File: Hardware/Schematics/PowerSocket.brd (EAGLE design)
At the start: 100 x 47.5 mm, 74 parts, among them T1 BT138-V, T2 BT138-V, T3 BT138-V, T4 BT138-V, T5 BT138-V, T6 BT138-V

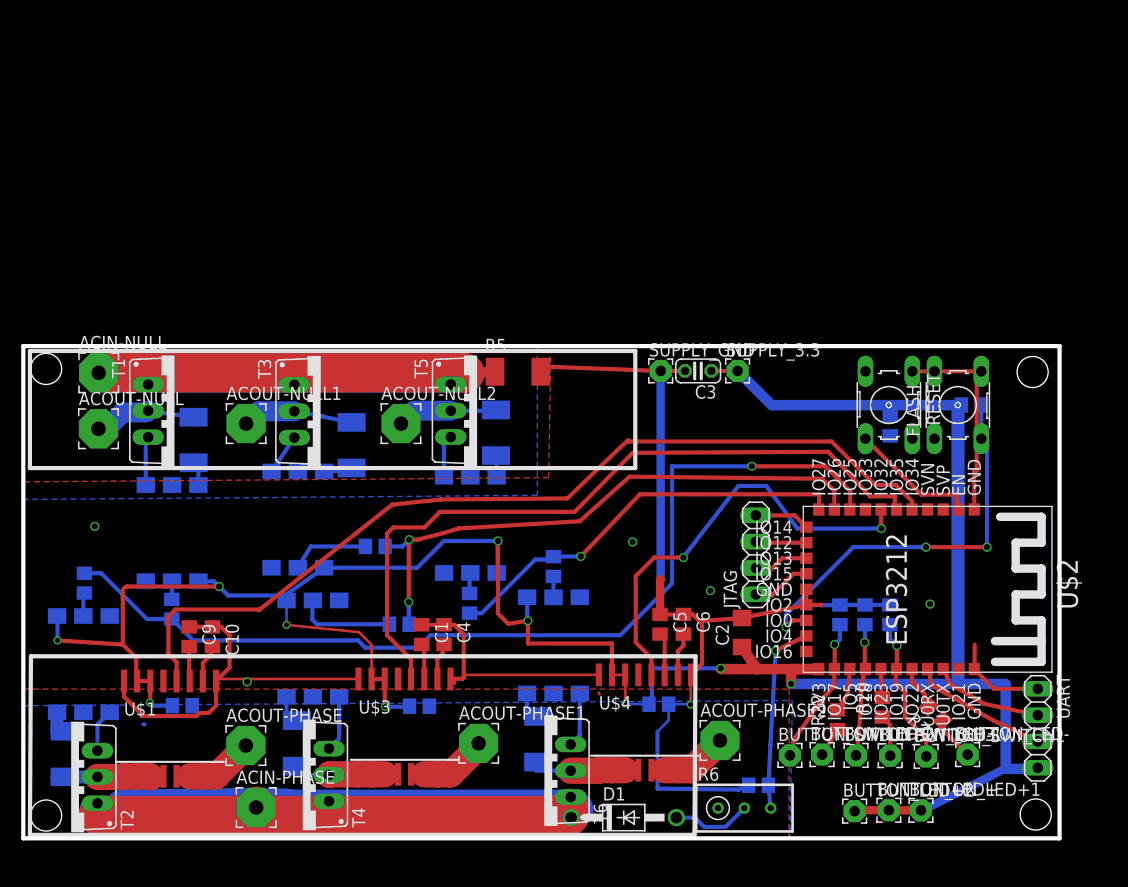
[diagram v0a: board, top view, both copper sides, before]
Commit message: New board layout
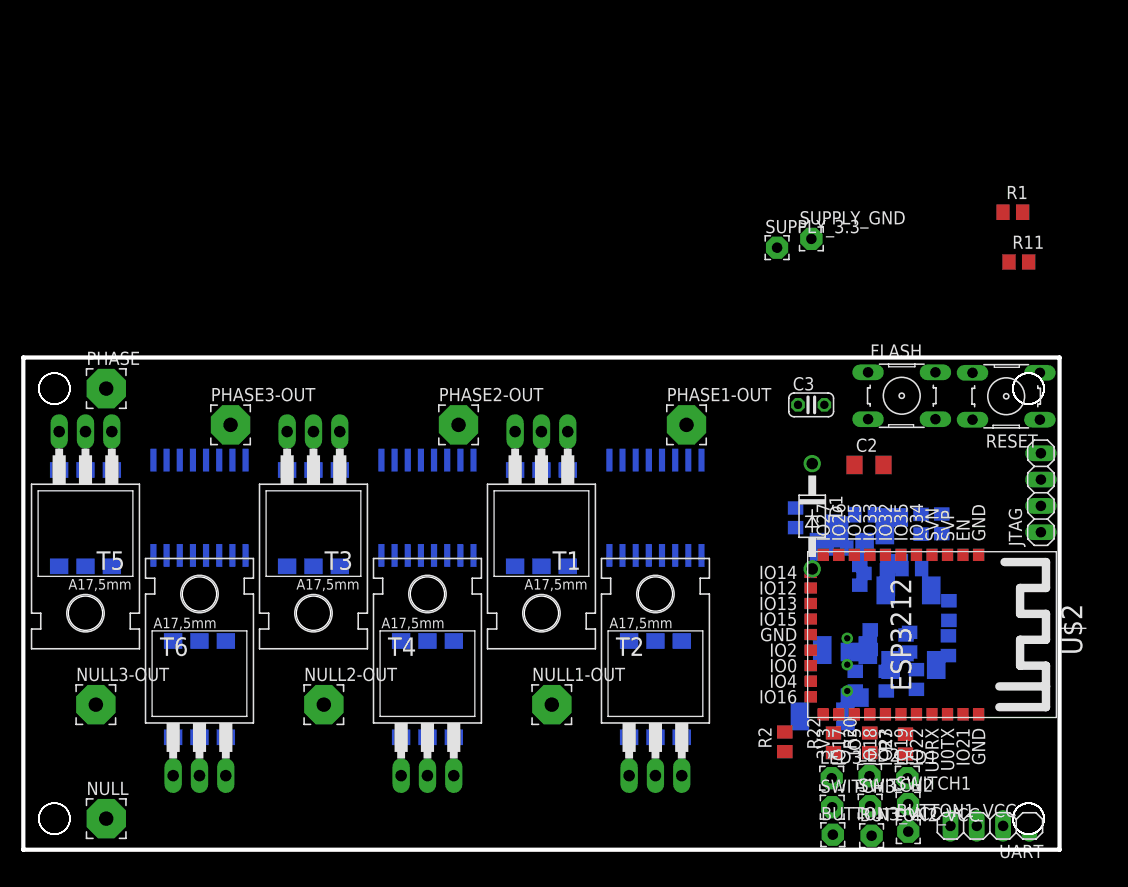
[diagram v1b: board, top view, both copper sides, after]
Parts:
- removed ACIN-NULL, ACIN-PHASE, ACOUT-NULL, ACOUT-NULL1, ACOUT-NULL2, ACOUT-PHASE, ACOUT-PHASE1, ACOUT-PHASE2: -, wirepad:3,81/1,4
- removed BUTTON_LED+: BUTTON_VCC, wirepad:2,15/1,0
- removed BUTTON_LED+1, BUTTON_LED+2, BUTTON_LED-, BUTTON_LED-1, BUTTON_LED-2, BUTTON_SWITCH1, BUTTON_SWITCH3, BUTTON_SWITCH5: -, wirepad:2,15/1,0
- removed U$1, U$3, U$4: ACS710, PowerSocket:SO-16DW
- added AMP1, AMP2, AMP3: ACS710, PowerSocket:SO-16DW
- added BUTTON1_VCC: (no value), wirepad:2,15/1,0
- added BUTTON2_VCC, BUTTON3_VCC, LED1, LED2, LED3, SWITCH1, SWITCH2, SWITCH3: -, wirepad:2,15/1,0
- added NULL, NULL1-OUT, NULL2-OUT, NULL3-OUT, PHASE, PHASE1-OUT, PHASE2-OUT, PHASE3-OUT: -, wirepad:3,81/1,4
- added R24: 0, eagle-ltspice:R2010
- R14, R18: device rcl:C0805 -> rcl:R0805
- T1, T2, T3, T4, T5, T6: value BT138-V -> BT138-H; device triac:TO220BV -> triac:TO220BH
- moved R9 83.6 mm to (89.3, 19.7), turned to 270 degrees
- moved R10 79.9 mm to (80.9, 30.8), turned to 180 degrees
- moved C11 71.6 mm to (85.7, 27.1)
- moved R3 69.1 mm to (83.4, 26.1)
- moved C10 67.3 mm to (85.5, 20.0), flipped to the bottom
- moved R4 66.1 mm to (79.3, 19.3), turned to 0 degrees
- moved C9 65.5 mm to (81.1, 27.6), flipped to the bottom
- moved T2 56.8 mm to (61.0, 13.5), turned to 0 degrees
- moved R11 56.4 mm to (96.1, 56.7), flipped to the top
- moved R15 55.9 mm to (79.0, 29.2), turned to 180 degrees
- moved R12 55.7 mm to (89.3, 23.1), turned to 270 degrees
- moved OK2 55.3 mm to (61.0, 15.5)
- moved R13 52.5 mm to (77.1, 12.9), turned to 0 degrees
- moved C1 49.3 mm to (86.6, 31.4), flipped to the bottom
- moved C4 49.2 mm to (88.6, 31.4), flipped to the bottom
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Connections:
- net N$25 renamed GATE2
- net N$3 renamed VOLTMETER
- removed net N$15 (its old number): BUTTON_LED-.1, R7.1
- removed net N$2 (its old number): R1.1, RESET.4, U$2.EN
- removed net N$36 (its old number): ACOUT-PHASE1.1, U$3.5, U$3.6, U$3.7, U$3.8
- removed net N$40: U$3.13
- removed net N$42 (its old number): OK5.2, R16.2
- removed net N$43: OK5.6, R17.1
- removed net N$45: ACIN-NULL.1, R5.1, T1.T1, T3.T1, T5.T1
- removed net N$46: OK6.2, R18.1
- removed net N$47: OK6.6, R19.1
- removed net N$49: R19.2, T6.T2, U$4.1, U$4.2, U$4.3, U$4.4
- removed net N$50: U$4.13
- removed net N$51: ACIN-PHASE.1, D1.C, T2.T1, T4.T1, T6.T1
- removed net N$52: R22.2, U$2.IO5
- removed net N$53: R15.2, T4.T2, U$3.1, U$3.2, U$3.3, U$3.4
- removed net N$54: R16.1, R18.2, U$2.IO27
- removed net N$55: C9.2, U$1.11
- removed net N$60: C10.2, U$1.10
- removed net N$62: C1.2, U$3.11
- removed net N$63: C4.2, U$3.10
- removed net N$64: C5.2, U$4.11
- removed net N$65: C6.2, U$4.10
- new net AMP1: AMP1.12, U$2.IO34
- new net AMP2: AMP2.12, U$2.IO35
- new net AMP3: AMP3.12, U$2.IO32
- new net BUTTON1: R8.1, SWITCH1.1, U$2.IO22
- new net BUTTON2: R21.1, SWITCH2.1, U$2.IO23
- new net BUTTON3: R23.1, SWITCH3.1, U$2.IO5
- new net GATE1: R3.2, R9.2, U$2.IO25
- new net GATE3: R16.1, R18.1, U$2.IO27
- new net LED1: R7.2, U$2.IO19
- new net LED2: R20.2, U$2.IO18
- new net LED3: R22.2, U$2.IO17
- new net N$24: FLASH.3, FLASH.4, R2.2, U$2.IO0
- new net N$30: AMP2.10, C4.1
- new net N$66: R1.1, RESET.3, RESET.4, U$2.EN
- new net NULL: NULL.1, R5.1, T2.T1, T4.T1, T6.T1
- new net PHASE: PHASE.1, R24.2, T1.T1, T3.T1, T5.T1
- new net PHASE1: AMP1.1, AMP1.2, AMP1.3, AMP1.4, R10.2, T1.T2
- new net PHASE2: AMP2.1, AMP2.2, AMP2.3, AMP2.4, R15.2, T3.T2
- new net PHASE3: AMP3.1, AMP3.2, AMP3.3, AMP3.4, R19.2, T5.T2
- net GND: now also AMP1.16, AMP1.9, AMP2.16, AMP2.9, AMP3.16, AMP3.9, C1.2, C10.2, C11.2, C12.2, C13.2, C4.2, C5.2, C6.2, C9.2, FLASH.1, R21.2, R23.2, R8.2, RESET.2; no longer C1.1, C10.1, C11.1, C12.1, C13.1, C4.1, C5.1, C6.1, C9.1, R21.1, R23.1, R8.1, U$1.16, U$1.9, U$3.16, U$3.9, U$4.16, U$4.9
- net N$1: now also OK1.2, R9.1; no longer ACOUT-NULL.1, R4.2, T1.T2
- net N$10: now also AMP3.5, AMP3.6, AMP3.7, AMP3.8, PHASE3-OUT.1; no longer OK2.2, R9.1
- net N$11: now also LED3.1, R22.1; no longer U$2.IO35, U$3.12
- net N$12: now also AMP1.10, C10.1; no longer U$1.12, U$2.IO34
- net N$13: now also AMP1.11, C9.1; no longer ACOUT-PHASE.1, U$1.5, U$1.6, U$1.7, U$1.8
- net N$14: now also NULL2-OUT.1, T4.T2; no longer ACOUT-NULL1.1, T3.T2
- net N$16: now also OK4.6, R13.1; no longer BUTTON_LED-1.1, R20.1
- net N$17: now also NULL1-OUT.1, R4.2, T2.T2; no longer BUTTON_SWITCH1.1, R8.2, U$2.IO19
- net N$18: now also OK5.2, R18.2; no longer OK1.6, R4.1
- net N$20: now also OK1.6, R10.1; no longer BUTTON_SWITCH3.1, R21.2, U$2.IO18
- net N$21: now also R4.1; no longer R10.1
- net N$23: now also OK3.6, R15.1; no longer R10.2, T2.T2, U$1.1, U$1.2, U$1.3, U$1.4
- net N$26: now also AMP2.5, AMP2.6, AMP2.7, AMP2.8, PHASE2-OUT.1; no longer BUTTON_LED-2.1, R22.1
- net N$27: now also AMP1.5, AMP1.6, AMP1.7, AMP1.8, PHASE1-OUT.1; no longer U$1.13
- net N$28: now also R14.1; no longer R12.2
- net N$29: now also OK4.2, R12.2; no longer OK3.6, R13.1
- net N$31: now also OK6.2, R16.2; no longer R20.2, U$2.IO23
- net N$32: now also AMP2.11, C1.1; no longer OK4.2, R14.1
- net N$33: now also OK6.6, R17.1; no longer OK4.6, R15.1
- net N$35: now also OK5.6, R19.1; no longer ACOUT-PHASE2.1, U$4.5, U$4.6, U$4.7, U$4.8
- net N$38: now also AMP3.10, C6.1; no longer ACOUT-NULL2.1, R17.2, T5.T2
- net N$39: now also AMP3.11, C5.1; no longer BUTTON_SWITCH5.1, R23.2, U$2.IO17
- net N$41: now also D1.C, R24.1; no longer U$2.IO32, U$4.12
- net N$6: now also OK2.2, R3.1; no longer OK1.2, R3.2
- net N$7: now also LED2.1, R20.1; no longer FLASH.3, R2.2, U$2.IO0
- net N$8: now also NULL3-OUT.1, R17.2, T6.T2; no longer R3.1, R9.2, U$2.IO25
- net N$9: now also LED1.1, R7.1; no longer R7.2, U$2.IO22
- net VCC: now also AMP1.14, AMP1.15, AMP2.14, AMP2.15, AMP3.14, AMP3.15, BUTTON1_VCC.1, BUTTON2_VCC.1, BUTTON3_VCC.1, C11.1, C12.1, C13.1; no longer BUTTON_LED+.1, BUTTON_LED+1.1, BUTTON_LED+2.1, C11.2, C12.2, C13.2, U$1.14, U$1.15, U$3.14, U$3.15, U$4.14, U$4.15
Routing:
- net VCC: track 252.8 -> 0.00 mm, vias 10 -> 0
- net GND: track 181.0 -> 0.00 mm, vias 6 -> 0
- net N$8: track 93.5 -> 0.00 mm, vias 1 -> 0
- net N$12: track 87.8 -> 0.00 mm
- net N$11: track 70.5 -> 0.00 mm
- net N$45: track 59.3 -> 0.00 mm
- net N$51: track 58.8 -> 0.00 mm
- net GATE2: track 55.9 -> 0.00 mm, vias 2 -> 0
- net N$68: track 47.4 -> 0.00 mm
- net N$41: track 41.9 -> 0.00 mm, vias 2 -> 0
- net N$54: track 40.1 -> 0.00 mm, vias 1 -> 0
- net N$7: track 39.8 -> 0.00 mm, vias 3 -> 0
- net N$37: track 34.3 -> 0.00 mm
- net VOLTMETER: track 18.5 -> 0.00 mm, vias 1 -> 0
- net N$17: track 14.2 -> 0.00 mm, vias 1 -> 0
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- removed copper zone on layer 1, net GND
- removed copper zone on layer 16, net GND

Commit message: Added .brd script.
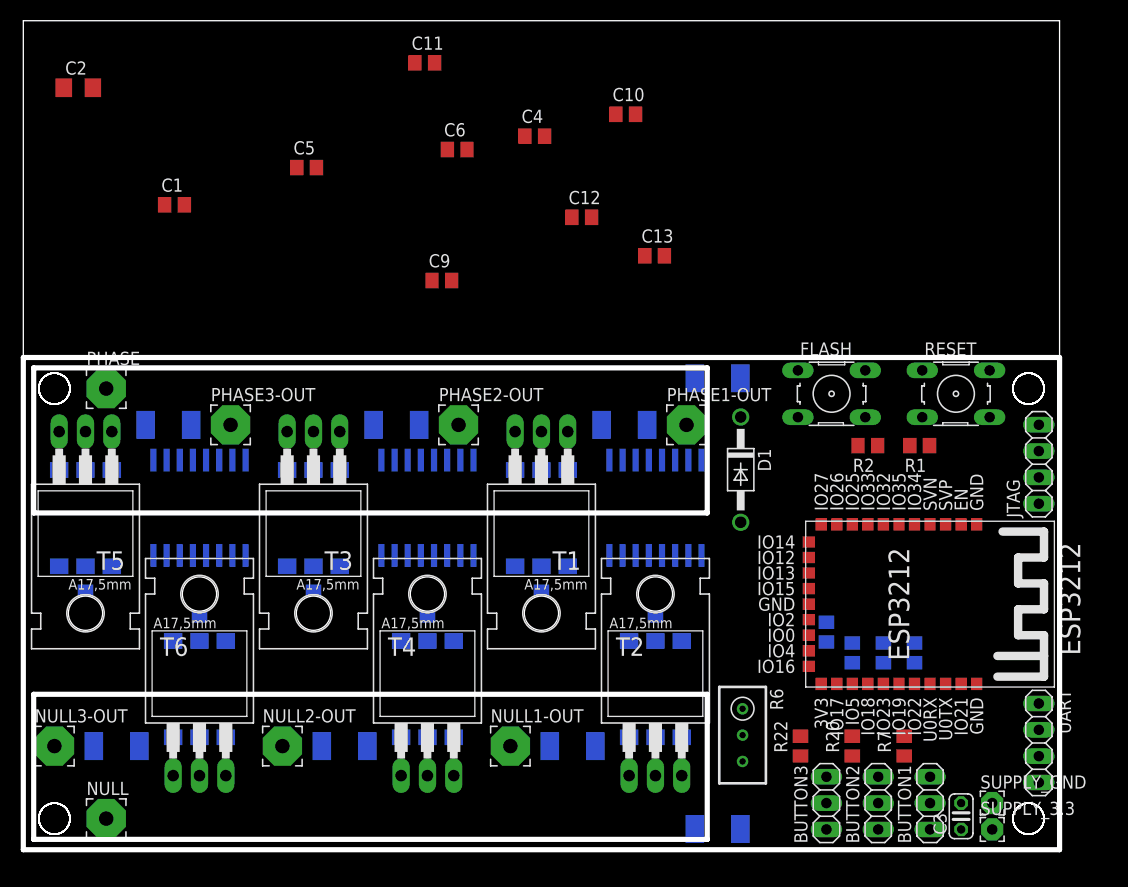
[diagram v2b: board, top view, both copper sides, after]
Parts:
- removed BUTTON1_VCC: (no value), wirepad:2,15/1,0
- removed BUTTON2_VCC, BUTTON3_VCC, LED1, LED2, LED3, SWITCH1, SWITCH2, SWITCH3: -, wirepad:2,15/1,0
- removed U$2: ESP3212LABELS, esp3212-ptw:ESP3212
- added BUTTON1, BUTTON2, BUTTON3: (no value), pinhead:1X03
- added ESP3212: ESP3212LABELS, esp3212-ptw:ESP3212
- moved C2 84.5 mm to (5.31, 73.5)
- moved R18 79.3 mm to (6.00, 24.0)
- moved C1 78.4 mm to (14.6, 62.2), flipped to the top, turned to 0 degrees
- moved R17 77.3 mm to (9.00, 10.0)
- moved R19 73.2 mm to (14.0, 41.0)
- moved C11 67.8 mm to (38.7, 75.9), flipped to the top
- moved R16 63.8 mm to (17.0, 23.5)
- moved C6 61.9 mm to (41.9, 67.6), flipped to the top, turned to 0 degrees
- moved C5 61.8 mm to (27.3, 65.8), flipped to the top, turned to 0 degrees
- moved SUPPLY_3.3 59.9 mm to (93.5, 1.96)
- moved C10 57.8 mm to (58.1, 71.0), flipped to the top, turned to 0 degrees
- moved SUPPLY_GND 57.2 mm to (93.5, 4.50)
- moved C4 54.3 mm to (49.4, 68.9), flipped to the top, turned to 0 degrees
- moved R12 50.3 mm to (39.0, 23.5)
- moved C9 49.1 mm to (40.4, 54.9), flipped to the top, turned to 0 degrees
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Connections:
- net AMP1: now also ESP3212.IO34; no longer U$2.IO34
- net AMP2: now also ESP3212.IO35; no longer U$2.IO35
- net AMP3: now also ESP3212.IO32; no longer U$2.IO32
- net BUTTON1: now also BUTTON1.3, ESP3212.IO22; no longer SWITCH1.1, U$2.IO22
- net BUTTON2: now also BUTTON2.3, ESP3212.IO23; no longer SWITCH2.1, U$2.IO23
- net BUTTON3: now also BUTTON3.3, ESP3212.IO5; no longer SWITCH3.1, U$2.IO5
- net GATE1: now also ESP3212.IO25; no longer U$2.IO25
- net GATE2: now also ESP3212.IO26; no longer U$2.IO26
- net GATE3: now also ESP3212.IO27; no longer U$2.IO27
- net GND: now also ESP3212.GND_B, ESP3212.GND_L, ESP3212.GND_R, ESP3212.IO2; no longer U$2.GND_B, U$2.GND_L, U$2.GND_R, U$2.IO2
- net LED1: now also ESP3212.IO19; no longer U$2.IO19
- net LED2: now also ESP3212.IO18; no longer U$2.IO18
- net LED3: now also ESP3212.IO17; no longer U$2.IO17
- net N$11: now also BUTTON3.2; no longer LED3.1
- net N$2: now also ESP3212.IO15; no longer U$2.IO15
- net N$24: now also ESP3212.IO0; no longer U$2.IO0
- net N$3: now also ESP3212.IO13; no longer U$2.IO13
- net N$4: now also ESP3212.IO12; no longer U$2.IO12
- net N$5: now also ESP3212.IO14; no longer U$2.IO14
- net N$66: now also ESP3212.EN; no longer U$2.EN
- net N$7: now also BUTTON2.2; no longer LED2.1
- net N$70: now also ESP3212.U0TX; no longer U$2.U0TX
- net N$77: now also ESP3212.U0RX; no longer U$2.U0RX
- net N$9: now also BUTTON1.2; no longer LED1.1
- net VCC: now also BUTTON1.1, BUTTON2.1, BUTTON3.1, ESP3212.3V3; no longer BUTTON1_VCC.1, BUTTON2_VCC.1, BUTTON3_VCC.1, U$2.3V3
- net VOLTMETER: now also ESP3212.IO4; no longer U$2.IO4
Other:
- board size 100 x 47.5 mm -> 100 x 80 mm
